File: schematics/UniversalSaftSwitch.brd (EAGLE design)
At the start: 53 x 35 mm, 20 parts, among them IC2 MAX485 CSA, IC3 AT90S2313S, K2 HF115F-024-S3, T1 BC817

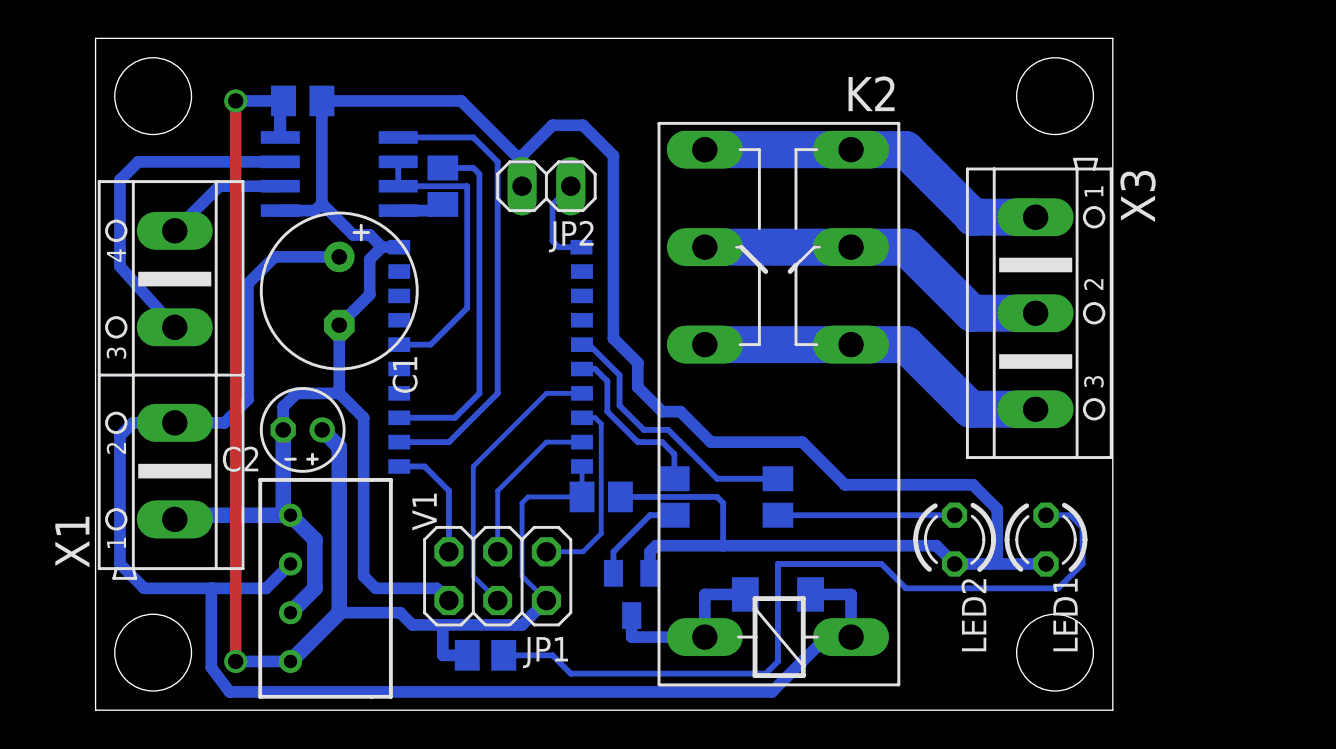
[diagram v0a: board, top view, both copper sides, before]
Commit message: New Schematic
Signed-off-by: Ralf Ramsauer <ralf@ramses-pyramidenbau.de>
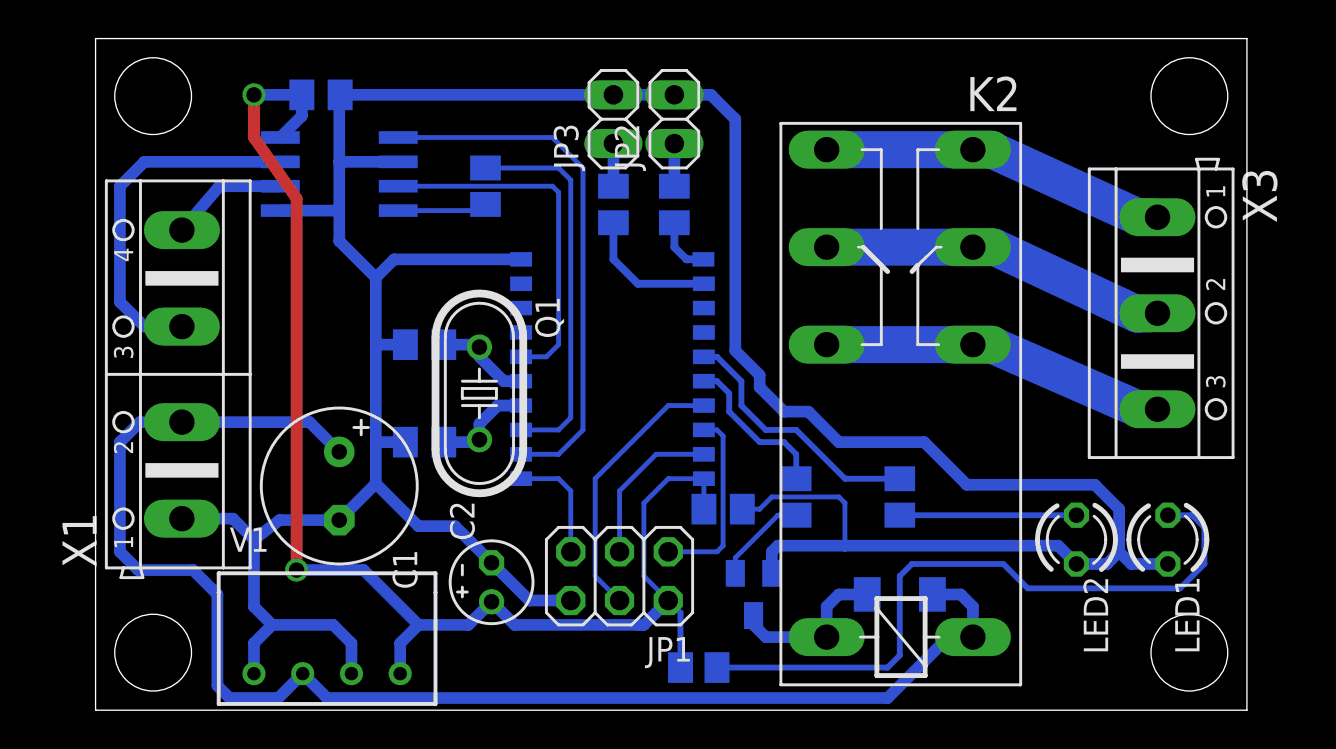
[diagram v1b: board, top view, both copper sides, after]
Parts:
- added C5, C6: 22p, rcl:C0805K
- added JP3: (no value), pinhead:1X02
- added Q1: 14.2, crystal:HC49U-V
- added R4, R6: 0, rcl:M0805
- moved C2 12.6 mm to (20.6, 6.67), turned to 90 degrees
- moved R1 11.1 mm to (31.4, 2.22)
- moved C1 10.2 mm to (12.7, 11.7)
- moved JP2 7.53 mm to (30.2, 30.8), turned to 90 degrees
- moved C3 6.38 mm to (32.7, 10.5)
- moved IC3 6.38 mm to (27.3, 17.1)
- moved JP1 6.35 mm to (27.3, 6.99)
- moved LED1 6.35 mm to (55.9, 8.89)
- moved LED2 6.35 mm to (51.1, 8.89)
- moved R5 6.35 mm to (36.5, 11.1)
- moved X3 6.35 mm to (55.3, 20.7)
- moved T1 6.35 mm to (34.3, 6.03)
- moved D2 6.35 mm to (41.9, 6.03)
- moved K2 6.35 mm to (41.9, 7.62)
- moved R2 6.35 mm to (41.9, 11.1)
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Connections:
- new net LED: IC3.12, R6.2
- new net N$10: C6.2, IC3.5, Q1.1
- new net N$11: JP2.1, R4.1
- new net N$12: JP3.1, R6.1
- new net N$7: C5.2, IC3.4, Q1.2
- net D+: now also IC2.6, X1.4; no longer IC2.7, X1.3
- net D-: now also IC2.7, X1.3; no longer IC2.6, X1.4
- net DE: no longer IC2.2
- net GND: now also C5.1, C6.1, IC2.2, JP3.2
- net PROG: now also R4.2; no longer JP2.1
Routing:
- net GND: track 145.2 -> 166.5 mm
- net D-: track 6.46 -> 18.7 mm
- net D+: track 17.5 -> 6.18 mm
- net LED: track 0.00 -> 7.15 mm
- net VCC: track 76.7 -> 70.6 mm
- net N$2: track 41.0 -> 35.2 mm
- net N$7: track 0.00 -> 5.30 mm
- net N$10: track 0.00 -> 5.12 mm
- net +24V: track 79.1 -> 74.9 mm
- net RXD: track 24.0 -> 27.7 mm
- net DE: track 15.5 -> 18.6 mm
- net N$1: track 2.40 -> 4.68 mm
- net N$12: track 0.00 -> 2.23 mm
- net N$11: track 0.00 -> 2.23 mm
- net PROG: track 4.89 -> 3.05 mm
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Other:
- board size 53 x 35 mm -> 60 x 35 mm
